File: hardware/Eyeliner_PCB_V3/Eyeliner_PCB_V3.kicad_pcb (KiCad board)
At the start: 2 copper layers, 0 parts

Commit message: Initial board bringup for v3.0
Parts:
- added Batt1: VBat, MountingHole:MountingHole_3.2mm_M3_DIN965_Pad, F.Cu at (156.5, 109.0)
- added C1: C0603X5R500-105KNP-CT, Capacitor_SMD:C_0603_1608Metric, B.Cu at (164.2, 97.7)
- added C10: 100 nF, Capacitor_SMD:C_0402_1005Metric, F.Cu at (162.7, 86.4)
- added C11: 100 nF, Capacitor_SMD:C_0402_1005Metric, B.Cu at (148.3, 80.7)
- added C12: 100 nF, Capacitor_SMD:C_0402_1005Metric, F.Cu at (162.7, 87.5)
- added C13: 100 nF, Capacitor_SMD:C_0402_1005Metric, F.Cu at (162.7, 85.3)
- added C14: 100 nF, Capacitor_SMD:C_0402_1005Metric, B.Cu at (156.7, 83.6)
- added C15: 100 nF, Capacitor_SMD:C_0402_1005Metric, B.Cu at (151.5, 97.5)
- added C16: 100 nF, Capacitor_SMD:C_0402_1005Metric, B.Cu at (157.4, 85.6)
- added C17: 1uF, Capacitor_SMD:C_0402_1005Metric, B.Cu at (160.1, 78.3)
- added C18: 100 nF, Capacitor_SMD:C_0402_1005Metric, B.Cu at (160.1, 79.5)
- added C19: GMC21X7R104K35NT, Capacitor_SMD:C_1206_3216Metric, B.Cu at (153.6, 97.4)
- added C2: 100nF, Capacitor_SMD:C_0402_1005Metric, B.Cu at (159.2, 94.2)
- added C20: GMT31X7R225K50NT2, Capacitor_SMD:C_1206_3216Metric, B.Cu at (155.9, 97.4)
- added C3: 16pF, Capacitor_SMD:C_0402_1005Metric, B.Cu at (161.1, 94.2)
- added C4: GMT32X7R106K35NT1, Capacitor_SMD:C_1210_3225Metric, F.Cu at (163.4, 90.4)
- added C5: 100 nF, Capacitor_SMD:C_0402_1005Metric, F.Cu at (150.9, 104.2)
- added C6: GMT32X7R106K35NT1, Capacitor_SMD:C_1210_3225Metric, B.Cu at (153.1, 102.1)
- added C7: GMT32X7R106K35NT1, Capacitor_SMD:C_1210_3225Metric, B.Cu at (159.7, 102.1)
- added C8: GMT32X7R106K35NT1, Capacitor_SMD:C_1210_3225Metric, B.Cu at (156.4, 102.1)
- added C9: GMT32X7R106K35NT1, Capacitor_SMD:C_1210_3225Metric, B.Cu at (149.8, 103.8)
- added D1: SPHV15-01ETG, Diode_SMD:D_SOD-882, F.Cu at (149.3, 99.4)
- added D2: STPS2L30A, Diode_SMD:D_SMA, B.Cu at (163.2, 80.6)
- added D3: SMAJ6.0A, Diode_SMD:D_SMA, F.Cu at (163.2, 81.2)
- added D4: RCLAMP03348P.U, RCLAMP03348P_U:TVS_RCLAMP03348P.U, B.Cu at (154.2, 93.4)
- added D5: SMAJ30A or SMAJ24A, Diode_SMD:D_SMA, B.Cu at (163.2, 103.5)
- added ESCs1: JST_SH_01x06, Connector_JST:JST_SH_SM06B-SRSS-TB_1x06-1MP_P1.00mm_Horizontal, B.Cu at (161.7, 89.2)
- added GND1: GND_ESCs, MountingHole:MountingHole_3.2mm_M3_DIN965_Pad, F.Cu at (161.9, 112.4)
- added HV1: HV_ESCs, MountingHole:MountingHole_3.2mm_M3_DIN965_Pad, F.Cu at (143.7, 112.4)
- added I2C1: JST_SH_01x04, Connector_JST:JST_SH_SM04B-SRSS-TB_1x04-1MP_P1.00mm_Horizontal, B.Cu at (146.2, 74.5)
- added J1: S7121-42R, S7121-42R:HARWIN_S7121-42R, F.Cu at (150.4, 108.5)
- added J3: SMTSO2020CTJ, MountingHole:SMTSO2020_Switch, B.Cu at (150.5, 112.2)
- added L1: SRP1038A-150M, Bourns_SRP1038A:IND_SRP1038A_BRN, F.Cu at (158.4, 100.3)
- added LEDs1: Conn_01x03_Pin, Connector_JST:JST_SH_SM03B-SRSS-TB_1x03-1MP_P1.00mm_Horizontal, B.Cu at (159.6, 74.5)
- added Q1: BSS138, Package_TO_SOT_SMD:SOT-323_SC-70, B.Cu at (155.6, 77.2)
- added Q2: IRFR9020PBF, Package_TO_SOT_SMD:TO-252-2, F.Cu at (144.9, 99.5)
- added R1: 100k, Resistor_SMD:R_0402_1005Metric, F.Cu at (150.6, 99.6)
- added R12: 100, Resistor_SMD:R_0402_1005Metric, F.Cu at (141.5, 86.8)
- added R13: 100, Resistor_SMD:R_0402_1005Metric, F.Cu at (141.6, 83.9)
- added R14: 100, Resistor_SMD:R_0402_1005Metric, B.Cu at (157.4, 84.6)
- added R15: 100, Resistor_SMD:R_0402_1005Metric, B.Cu at (148.9, 100.5)
- added R16: 100, Resistor_SMD:R_0402_1005Metric, B.Cu at (148.9, 99.5)
- added R17: 100, Resistor_SMD:R_0402_1005Metric, B.Cu at (148.9, 98.5)
- added R18: 100, Resistor_SMD:R_0402_1005Metric, F.Cu at (152.2, 95.8)
- added R19: 1k, Resistor_SMD:R_0402_1005Metric, B.Cu at (153.5, 77.8)
- added R2: 32.4k, Resistor_SMD:R_0402_1005Metric, B.Cu at (162.4, 99.5)
- added R20: 1k, Resistor_SMD:R_0402_1005Metric, B.Cu at (155.4, 75.5)
- added R21: 100, Resistor_SMD:R_0402_1005Metric, B.Cu at (157.4, 78.4)
- added R22: 100, Resistor_SMD:R_0402_1005Metric, B.Cu at (157.4, 91.7)
- added R23: 100, Resistor_SMD:R_0402_1005Metric, B.Cu at (157.4, 90.7)
- added R24: 100, Resistor_SMD:R_0402_1005Metric, B.Cu at (157.4, 88.7)
- added R25: 100, Resistor_SMD:R_0402_1005Metric, B.Cu at (157.4, 87.7)
- added R26: 4.7k, Resistor_SMD:R_0402_1005Metric, B.Cu at (147.8, 79.2)
- added R27: 4.7k, Resistor_SMD:R_0402_1005Metric, B.Cu at (143.3, 82.5)
- added R28: 4.7k, Resistor_SMD:R_0402_1005Metric, F.Cu at (141.6, 76.1)
- added R29: 4.7k, Resistor_SMD:R_0402_1005Metric, B.Cu at (141.8, 78.1)
- added R3: 20k, Resistor_SMD:R_0402_1005Metric, B.Cu at (163.9, 95.2)
- added R30: 100, Resistor_SMD:R_0402_1005Metric, B.Cu at (141.9, 76.1)
- added R31: 100, Resistor_SMD:R_0402_1005Metric, B.Cu at (142.9, 77.8)
- added R4: 5.1k, Resistor_SMD:R_0402_1005Metric, F.Cu at (164.1, 93.7)
- added R5: 1k, Resistor_SMD:R_0402_1005Metric, F.Cu at (162.5, 94.2)
- added R6: 22k, Resistor_SMD:R_0402_1005Metric, F.Cu at (149.9, 105.2)
- added R7: 2k, Resistor_SMD:R_0402_1005Metric, F.Cu at (141.5, 88.8)
- added R8: RC1206FR-07100RL, Resistor_SMD:R_1206_3216Metric, F.Cu at (142.9, 107.2)
- added R9: 4.7k, Resistor_SMD:R_0402_1005Metric, F.Cu at (141.8, 81.5)
- added Receiver1: ~, Stuff from Walnut:BetaFPV ELRS Lite, B.Cu at (145.2, 91.7)
- added Temps1: JST_SH_01x04, Connector_JST:JST_SH_SM04B-SRSS-TB_1x04-1MP_P1.00mm_Horizontal, B.Cu at (144.5, 100.0)
- added U1: LM61440AANRJRR, LM61440:LM61440AASQRJRRQ1, B.Cu at (160.8, 96.8)
- added U2: XIAO-ESP32-S3-SMD, Seeed_Studio_XIAO_Series:XIAO-ESP32-S3-SMD_Minimal, F.Cu at (142.9, 94.7)
- added U3: TMUX154ERSW, Package_DFN_QFN:UQFN-10_1.4x1.8mm_P0.4mm, B.Cu at (143.1, 80.1)
- added U4: LSM6DSV320XTR, Package_LGA:LGA-14_3x2.5mm_P0.5mm_LayoutBorder3x4y, B.Cu at (146.2, 82.2)
- added U5: LSM6DSV320XTR, Package_LGA:LGA-14_3x2.5mm_P0.5mm_LayoutBorder3x4y, B.Cu at (159.1, 82.2)
- added U6: TMUX1204DQAR, Package_SON:USON-10_2.5x1.0mm_P0.5mm, F.Cu at (150.6, 96.3)
- added U7: RCLAMP3346P.TNT, RCLAMP3346P:SGP2708N7_SEM, B.Cu at (150.4, 77.8)
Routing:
- net VCC_3V3: track 0.00 -> 88.6 mm, vias 0 -> 13
- net /Top_Board/Vbat_Sense: track 0.00 -> 48.2 mm, vias 0 -> 3
- net /Top_Board/Temp_Sense: track 0.00 -> 47.8 mm, vias 0 -> 1
- net VCC_5V: track 0.00 -> 40.7 mm, vias 0 -> 7
- net VCC_HV: track 0.00 -> 35.2 mm, vias 0 -> 35
- net /Top_Board/Bias: track 0.00 -> 34.9 mm, vias 0 -> 2
- net GND: track 0.00 -> 27.1 mm, vias 0 -> 48
- net /Top_Board/SCL_Accel: track 0.00 -> 24.8 mm
- net /Top_Board/INT: track 0.00 -> 24.6 mm, vias 0 -> 2
- net /Top_Board/Receiver_TX: track 0.00 -> 22.1 mm, vias 0 -> 3
- net /Top_Board/SDA_Accel: track 0.00 -> 20.5 mm
- net /Top_Board/ESC_Telem1: track 0.00 -> 18.0 mm, vias 0 -> 1
- net /Top_Board/ESC_Telem2: track 0.00 -> 15.9 mm, vias 0 -> 1
- net /Top_Board/Temp_Sel2: track 0.00 -> 15.8 mm
- net /Top_Board/SDA_Extra: track 0.00 -> 14.8 mm, vias 0 -> 1
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- added copper zone on B.Cu, net GND
- added copper zone on F.Cu, net GND
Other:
- board outline added: 25.4 x 44.6 mm

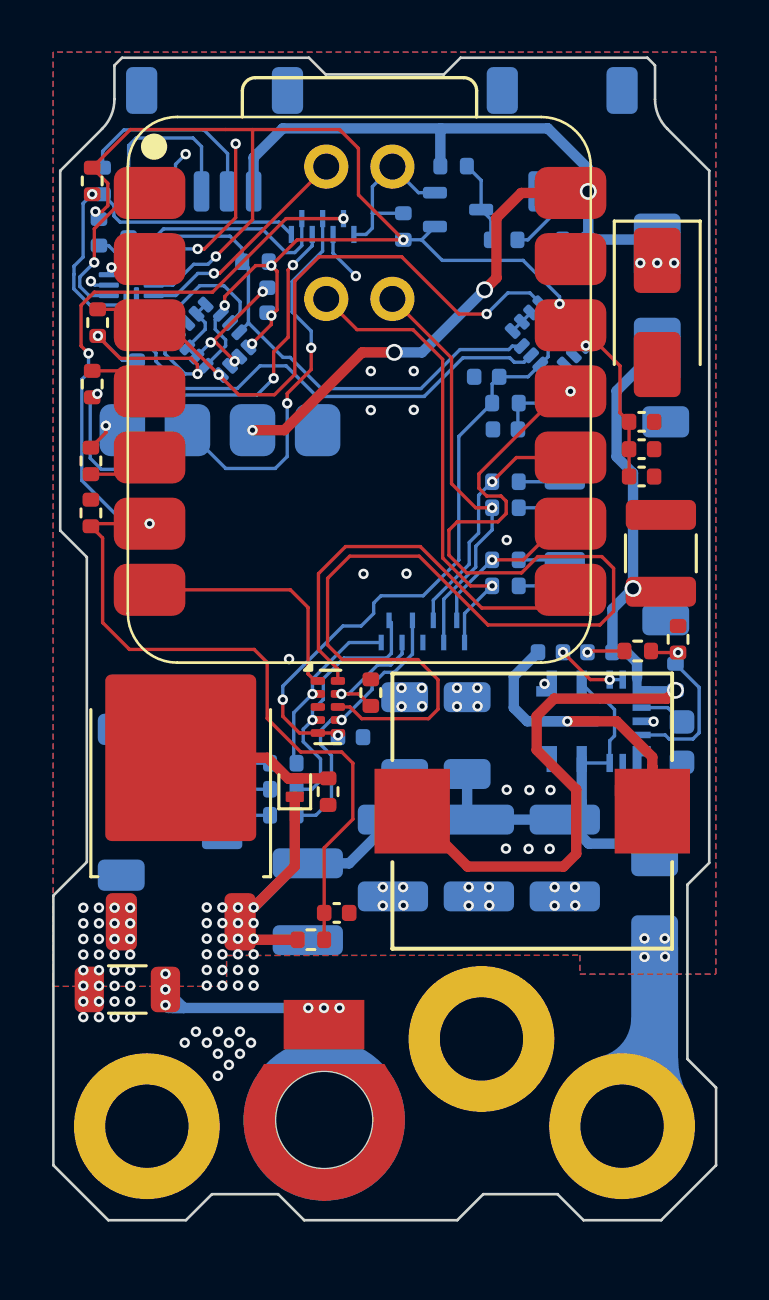
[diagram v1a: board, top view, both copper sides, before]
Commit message: All basic board functionality working
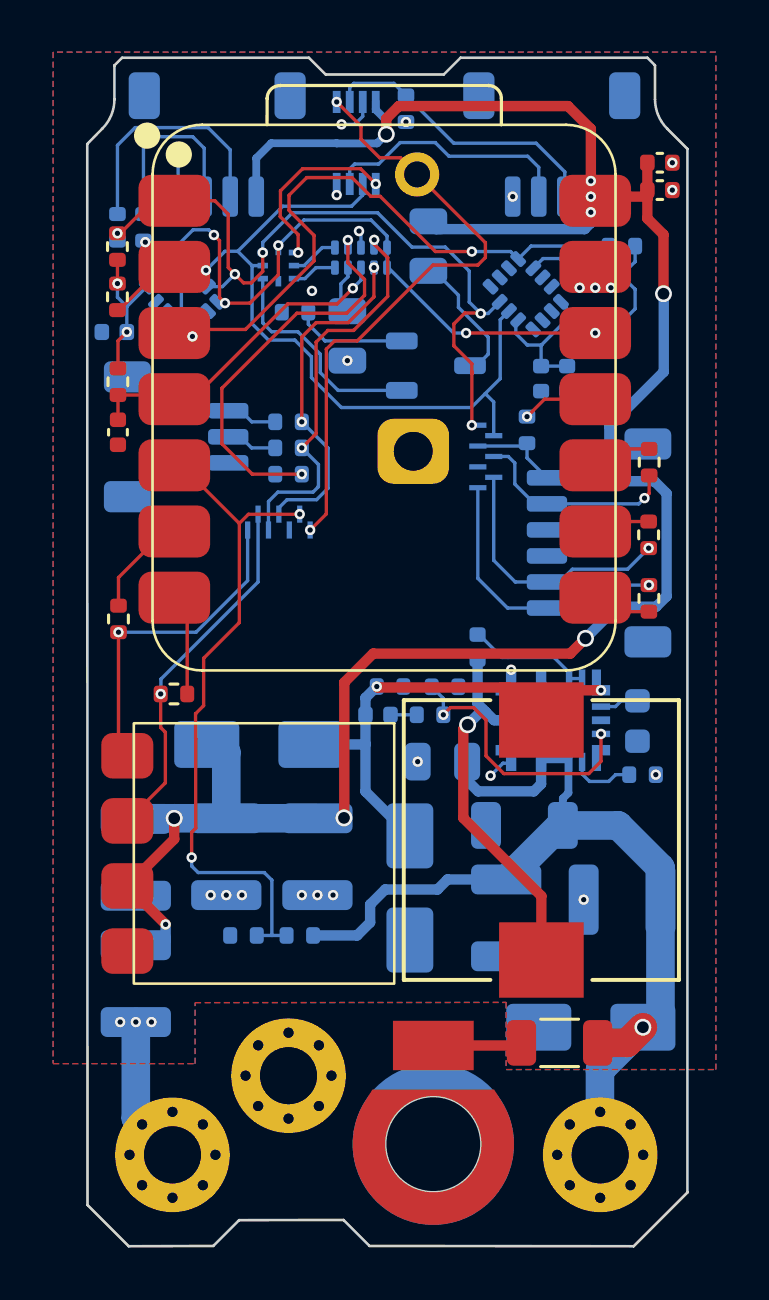
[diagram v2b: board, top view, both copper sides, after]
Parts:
- removed C18: 100 nF, Capacitor_SMD:C_0402_1005Metric
- removed C19: GMC21X7R104K35NT, Capacitor_SMD:C_1206_3216Metric
- removed C20: GMT31X7R225K50NT2, Capacitor_SMD:C_1206_3216Metric
- removed D4: RCLAMP03348P.U, RCLAMP03348P_U:TVS_RCLAMP03348P.U
- removed D5: SMAJ30A or SMAJ24A, Diode_SMD:D_SMA
- removed J3: SMTSO2020CTJ, MountingHole:SMTSO2020_Switch
- removed LEDs1: Conn_01x03_Pin, Connector_JST:JST_SH_SM03B-SRSS-TB_1x03-1MP_P1.00mm_Horizontal
- removed Q2: IRFR9020PBF, Package_TO_SOT_SMD:TO-252-2
- removed R25, R30, R31: 100, Resistor_SMD:R_0402_1005Metric
- removed R26, R27, R28, R29: 4.7k, Resistor_SMD:R_0402_1005Metric
- removed the U3 at (143.1, 80.1)
- added Conn_LEDs1: JST_SH_01x04, Connector_JST:JST_SH_SM04B-SRSS-TB_1x04-1MP_P1.00mm_Horizontal, B.Cu at (159.2, 74.7)
- added IC1: PCA9570GMH, PCA9570:PCA9570GMH, B.Cu at (148.7, 79.3)
- added IC2: 74AHCT2G125DC,125, 74AHCT2G125DC, 125:SOP50P310X100-8N, B.Cu at (151.7, 74.6)
- added IR1: TestPoint_2Pole, Capacitor_SMD:C_0805_2012Metric, B.Cu at (154.5, 78.6)
- added J2: 4871, MountingHole:4871_Switch_Precharge, F.Cu at (154.7, 113.1)
- added R10: 1k, Resistor_SMD:R_0402_1005Metric, F.Cu at (142.5, 80.5)
- added R11: 20k, Resistor_SMD:R_0402_1005Metric, B.Cu at (149.5, 105.1)
- added RTD_Onboard1: TestPoint_2Pole, Capacitor_SMD:C_0805_2012Metric, B.Cu at (151.3, 82.0)
- added U5: TMUX1204DQAR, Package_SON:USON-10_2.5x1.0mm_P0.5mm, B.Cu at (151.9, 79.0)
- Batt1, GND1, HV1: footprint MountingHole:MountingHole_3.2mm_M3_DIN965_Pad -> MountingHole:MountingHole_2.2mm_M2_Pad_Via
- C10: value 100 nF -> 16pF; moved to B.Cu
- C11, C16: value 100 nF -> MSASG32MSB5226MPNA01; footprint Capacitor_SMD:C_0402_1005Metric -> Capacitor_SMD:C_1210_3225Metric
- C12, C5: value 100 nF -> MSASG32MSB5226MPNA01; footprint Capacitor_SMD:C_0402_1005Metric -> Capacitor_SMD:C_1210_3225Metric; moved to B.Cu
- C13: value 100 nF -> 1uF
- C14, C15, R21, R22, R23, Receiver1: moved to F.Cu
- C17: value 1uF -> MSASG32MSB5226MPNA01; footprint Capacitor_SMD:C_0402_1005Metric -> Capacitor_SMD:C_1210_3225Metric
- C2: value 100nF -> GMC21X7R104K35NT; footprint Capacitor_SMD:C_0402_1005Metric -> Capacitor_SMD:C_0805_2012Metric
- C3: value 16pF -> MSASG32MSB5226MPNA01; footprint Capacitor_SMD:C_0402_1005Metric -> Capacitor_SMD:C_1210_3225Metric
- C4: value GMT32X7R106K35NT1 -> GCJ31CR71H225KA12L; footprint Capacitor_SMD:C_1210_3225Metric -> Capacitor_SMD:C_1206_3216Metric; moved to B.Cu
- C6: value GMT32X7R106K35NT1 -> 470nF; footprint Capacitor_SMD:C_1210_3225Metric -> Capacitor_SMD:C_0402_1005Metric
- C7: value GMT32X7R106K35NT1 -> 100nF; footprint Capacitor_SMD:C_1210_3225Metric -> Capacitor_SMD:C_0402_1005Metric
- C8, C9: value GMT32X7R106K35NT1 -> 100 nF; footprint Capacitor_SMD:C_1210_3225Metric -> Capacitor_SMD:C_0402_1005Metric
- D1: value SPHV15-01ETG -> SMAJ30A or SMAJ24A; footprint Diode_SMD:D_SOD-882 -> Diode_SMD:D_SMA; moved to B.Cu
- D2: value STPS2L30A -> SMAJ6.0A
- D3: value SMAJ6.0A -> STPS2L30A; moved to B.Cu
- J1: value S7121-42R -> S7131-45R
- Q1: footprint Package_TO_SOT_SMD:SOT-323_SC-70 -> Package_TO_SOT_SMD:TSOT-23
- R1: value 100k -> 4.7k; moved to B.Cu
- R12: value 100 -> 2k; moved to B.Cu
- R13: value 100 -> 1k
- R14: value 100 -> 1k; moved to F.Cu
- R18: moved to B.Cu
- R19: value 1k -> 4.7k
- R2: value 32.4k -> 100; moved to F.Cu
- R20: value 1k -> 100
- R24: value 100 -> 10k
- R3: value 20k -> 100; moved to F.Cu
- R4: value 5.1k -> 30k; moved to B.Cu
- R5: value 1k -> 100; moved to B.Cu
- R6: value 22k -> RC1206FR-07100RL; footprint Resistor_SMD:R_0402_1005Metric -> Resistor_SMD:R_1206_3216Metric
- R7: value 2k -> 20k; moved to B.Cu
- R8: value RC1206FR-07100RL -> 5.1k; footprint Resistor_SMD:R_1206_3216Metric -> Resistor_SMD:R_0402_1005Metric; moved to B.Cu
- R9: value 4.7k -> 1k; moved to B.Cu
- Temps1: value JST_SH_01x04 -> JST_SH_01x03; footprint Connector_JST:JST_SH_SM04B-SRSS-TB_1x04-1MP_P1.00mm_Horizontal -> Connector_JST:JST_SH_SM03B-SRSS-TB_1x03-1MP_P1.00mm_Horizontal
- U2: footprint Seeed_Studio_XIAO_Series:XIAO-ESP32-S3-SMD_Minimal -> Seeed_Studio_XIAO_Series:XIAO-ESP32-S3-SMD
- U6: value TMUX1204DQAR -> RCLAMP3346P.TNT; footprint Package_SON:USON-10_2.5x1.0mm_P0.5mm -> RCLAMP3346P:SGP2708N7_SEM; moved to B.Cu
- moved C17 33.2 mm to (143.2, 106.9), turned to -90 degrees
- moved C8 24.6 mm to (142.4, 81.9), turned to 180 degrees
- moved D2 24.6 mm to (153.8, 103.2)
- moved R1 23.8 mm to (161.9, 78.6), turned to 0 degrees
- moved R15 23.2 mm to (143.5, 77.9), turned to 90 degrees
- moved D3 22.6 mm to (147.9, 97.7), turned to 0 degrees
- moved R16 22.5 mm to (142.5, 77.9), turned to -90 degrees
- moved C9 22.4 mm to (159.8, 83.7)
- moved C16 21.7 mm to (143.2, 102.1), turned to -90 degrees
- moved R3 21.5 mm to (142.6, 92.9), turned to 90 degrees
- moved C11 21.4 mm to (146.7, 102.0), turned to -90 degrees
- moved R9 19.7 mm to (154.5, 96.6), turned to 0 degrees
- moved C6 19.3 mm to (158.8, 83.7)
- moved C12 19.2 mm to (150.2, 102.0), turned to -90 degrees
- moved R12 19.1 mm to (147.4, 105.1), turned to 0 degrees
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- renumbered U4 to U3, U5 to U4
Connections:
- C10 pad 1: VCC_3V3 -> /Top_Board/Bias
- C10 pad 2: GND -> Net-(C10-Pad2)
- C11 pad 1: VCC_3V3 -> VCC_5V
- C12 pad 1: VCC_3V3 -> VCC_5V
- C13 pad 1: VCC_3V3 -> VCC_5V
- C14 pad 1: VCC_3V3 -> VCC_5V
- C15 pad 1: VCC_3V3 -> /Top_Board/Sense
- C16 pad 1: /Top_Board/Temp_Sense -> VCC_5V
- C2 pad 1: Net-(U1-SW) -> VCC_HV
- C2 pad 2: Net-(U1-CBOOT) -> GND
- C3 pad 1: /Top_Board/Bias -> VCC_HV
- C3 pad 2: Net-(C3-Pad2) -> GND
- C4 pad 1: /Top_Board/Bias -> VCC_HV
- C5 pad 1: /Top_Board/Vbat_Sense -> VCC_HV
- C6 pad 1: VCC_HV -> VCC_3V3
- C7 pad 1: VCC_HV -> Net-(U1-SW)
- C7 pad 2: GND -> Net-(U1-CBOOT)
- C8 pad 1: VCC_HV -> VCC_3V3
- C9 pad 1: VCC_HV -> VCC_3V3
- D1 pad 2: Net-(D1-A) -> GND
- D2 pad 1: VCC_5V -> /Top_Board/Bias
- D2 pad 2: /Top_Board/Bias -> GND
- D3 pad 2: GND -> /Top_Board/Bias
- ESCs1 pad 1: GND -> /Top_Board/ESC_Telem2_Proc
- ESCs1 pad 2: Net-(ESCs1-Pin_2) -> /Top_Board/Dshot2_Proc
- ESCs1 pad 3: Net-(ESCs1-Pin_3) -> GND
- ESCs1 pad 5: Net-(ESCs1-Pin_5) -> /Top_Board/Dshot1_Proc
- ESCs1 pad 6: Net-(ESCs1-Pin_6) -> /Top_Board/ESC_Telem1_Proc
- ESCs1 pad MP: (no net) -> GND
- I2C1 pad MP: (no net) -> GND
- Q1 pad 1: VCC_3V3 -> Net-(IC1-P3)
- Q1 pad 2: /Top_Board/LEDs -> Net-(Q1-S)
- R1 pad 1: Net-(D1-A) -> /Top_Board/INT
- R1 pad 2: GND -> VCC_3V3
- R12 pad 1: /Top_Board/Receiver_RX -> GND
- R12 pad 2: Net-(U2-D4) -> /Top_Board/Vbat_Sense
- R13 pad 1: Net-(U2-D3) -> /Top_Board/SDA
- R13 pad 2: /Top_Board/Receiver_TX -> VCC_3V3
- R14 pad 1: /Top_Board/Temp_Sense -> /Top_Board/Sense
- R15 pad 1: Net-(Temps1-Pin_2) -> /Top_Board/SCL
- R15 pad 2: /Top_Board/Temp1_1 -> Net-(I2C1-Pin_2)
- R16 pad 1: Net-(Temps1-Pin_3) -> Net-(I2C1-Pin_3)
- R16 pad 2: /Top_Board/Temp2_1 -> /Top_Board/SDA
- R17 pad 1: Net-(Temps1-Pin_4) -> Net-(Temps1-Pin_2)
- R17 pad 2: /Top_Board/Temp3_1 -> /Top_Board/Temp2_1
- R18 pad 1: GND -> Net-(Temps1-Pin_3)
- R18 pad 2: /Top_Board/TempRef_1 -> /Top_Board/Temp1_1
- R19 pad 1: VCC_3V3 -> GND
- R19 pad 2: /Top_Board/LEDs -> /Top_Board/TempRef_1
- R2 pad 1: GND -> Net-(U2-D6)
- R2 pad 2: Net-(U1-RT) -> /Top_Board/Receiver_TX
- R20 pad 1: VCC_5V -> /Top_Board/ESC_Telem2_Proc
- R20 pad 2: Net-(Q1-D) -> /Top_Board/ESC_Telem2
- R21 pad 1: Net-(LEDs1-Pin_2) -> /Top_Board/Dshot2_Proc
- R21 pad 2: Net-(Q1-D) -> /Top_Board/Dshot2
- R22 pad 1: Net-(ESCs1-Pin_6) -> /Top_Board/ESC_Telem1_Proc
- R23 pad 1: Net-(ESCs1-Pin_5) -> /Top_Board/Dshot1_Proc
- R24 pad 1: Net-(ESCs1-Pin_3) -> GND
- R24 pad 2: /Top_Board/ESC_Telem2 -> Net-(Conn_LEDs1-Pin_3)
- R3 pad 1: /Top_Board/FB -> /Top_Board/Receiver_RX
- R3 pad 2: /Top_Board/Bias -> Net-(U2-D5)
- R4 pad 2: /Top_Board/FB -> Net-(U1-RT)
- R5 pad 1: Net-(C3-Pad2) -> GND
- R5 pad 2: /Top_Board/FB -> Net-(Q1-S)
- R6 pad 1: /Top_Board/Vbat_Sense -> VCC_HV
- R6 pad 2: VCC_HV -> Net-(J1-SHIELD)
- R7 pad 1: GND -> /Top_Board/FB
- R7 pad 2: /Top_Board/Vbat_Sense -> /Top_Board/Bias
- R8 pad 1: VCC_NoProc -> GND
- R8 pad 2: Net-(J1-SHIELD) -> /Top_Board/FB
- R9 pad 1: /Top_Board/INT -> Net-(C10-Pad2)
- R9 pad 2: VCC_3V3 -> /Top_Board/FB
- Temps1 pad MP: (no net) -> GND
- U2 pad 11: /Top_Board/Temp_Sense -> /Top_Board/ESC_Telem2
- U2 pad 4: Net-(U2-D3) -> /Top_Board/Sense
- U2 pad 5: Net-(U2-D4) -> /Top_Board/Vbat_Sense
- U2 pad 6: /Top_Board/Vbat_Sense -> Net-(U2-D5)
- U2 pad 7: /Top_Board/Temp_Sel1 -> Net-(U2-D6)
- U2 pad 8: /Top_Board/Temp_Sel2 -> /Top_Board/ESC_Telem1
- U3 pad 13: /Top_Board/SCL_Accel -> /Top_Board/SCL
- U3 pad 14: /Top_Board/SDA_Accel -> /Top_Board/SDA
- U4 pad 13: /Top_Board/SCL_Accel -> /Top_Board/SCL
- U4 pad 14: /Top_Board/SDA_Accel -> /Top_Board/SDA
- U6 pad 1: /Top_Board/Temp_Sel1 -> /Top_Board/LEDs
- U6 pad 2: /Top_Board/Temp3_1 -> GND
- U6 pad 3: GND -> /Top_Board/Temp2_1
- U6 pad 4: /Top_Board/Temp2_1 -> /Top_Board/Receiver_RX
- U6 pad 5: VCC_3V3 -> /Top_Board/Receiver_TX
- U6 pad 6: VCC_3V3 -> /Top_Board/Temp1_1
- U6 pad 7: /Top_Board/Temp1_1 -> /Top_Board/Vbat_Sense
- U7 pad 1: /Top_Board/LEDs -> /Top_Board/ESC_Telem1_Proc
- U7 pad 3: /Top_Board/Receiver_RX -> /Top_Board/ESC_Telem2_Proc
- U7 pad 4: /Top_Board/SDA_Extra -> /Top_Board/SDA
- U7 pad 5: /Top_Board/SCL_Extra -> /Top_Board/SCL
- U7 pad 6: /Top_Board/Receiver_TX -> /Top_Board/Dshot2_Proc
- U7 pad 7: /Top_Board/Vbat_Sense -> /Top_Board/Dshot1_Proc
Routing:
- net /Top_Board/Temp_Sense: track 47.8 -> 0.00 mm, vias 1 -> 0
- net VCC_5V: track 40.7 -> 83.5 mm, vias 7 -> 9
- net VCC_3V3: track 88.6 -> 49.7 mm, vias 13 -> 7
- net /Top_Board/SCL: track 1.92 -> 30.2 mm, vias 1 -> 2
- net /Top_Board/SCL_Accel: track 24.8 -> 0.00 mm
- net /Top_Board/SDA: track 6.39 -> 29.0 mm, vias 1 -> 5
- net /Top_Board/Vbat_Sense: track 48.2 -> 26.4 mm, vias 3 -> 2
- net /Top_Board/SDA_Accel: track 20.5 -> 0.00 mm
- net /Top_Board/Bias: track 34.9 -> 16.3 mm
- net /Top_Board/LEDs: track 6.73 -> 23.6 mm, vias 0 -> 2
- net GND: track 27.1 -> 10.5 mm, vias 48 -> 27
- net /Top_Board/ESC_Telem1: track 18.0 -> 2.28 mm, vias 1 -> 0
- net /Top_Board/SDA_Extra: track 14.8 -> 0.00 mm, vias 1 -> 0
- net /Top_Board/Temp_Sel2: track 15.8 -> 1.75 mm
- net /Top_Board/ESC_Telem2: track 15.9 -> 2.90 mm
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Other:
- board size 25.4 x 44.6 mm -> 23 x 45.6 mm
